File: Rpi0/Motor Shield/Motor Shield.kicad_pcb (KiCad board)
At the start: 2 copper layers, 29.8 x 64.8 mm, 37 parts, among them J1 Screw_Terminal_01x02, J3 Conn_02x01, J4 Screw_Terminal_01x02, J5 Screw_Terminal_01x02, J6 Conn_01x04_Female, J7 Conn_01x04_Female, Q1 Q_PMOS_GDSD, U1 IFX9201SG, U2 IFX9201SG, U3 PIC16F1509-ISS, U4 RPI0-Template, U6 ACT4060A

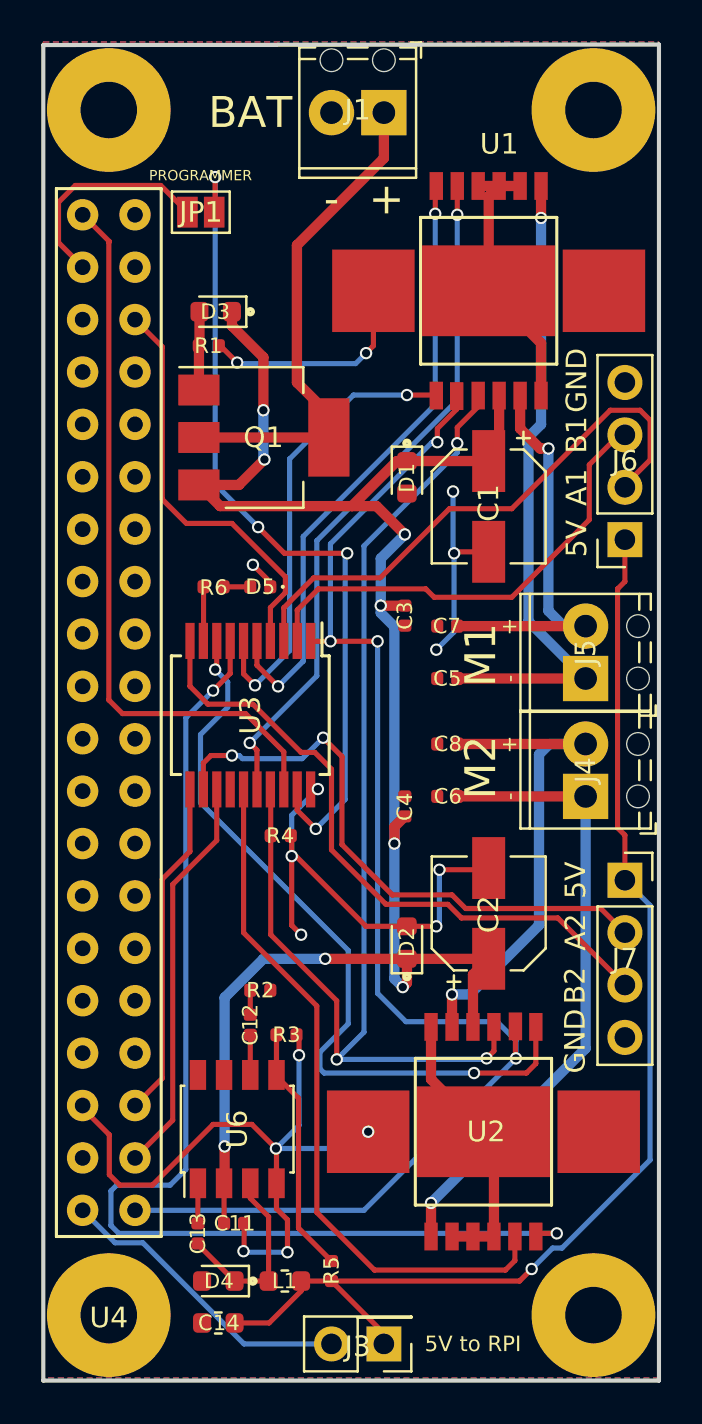
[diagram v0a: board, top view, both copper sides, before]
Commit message: Changed footprint
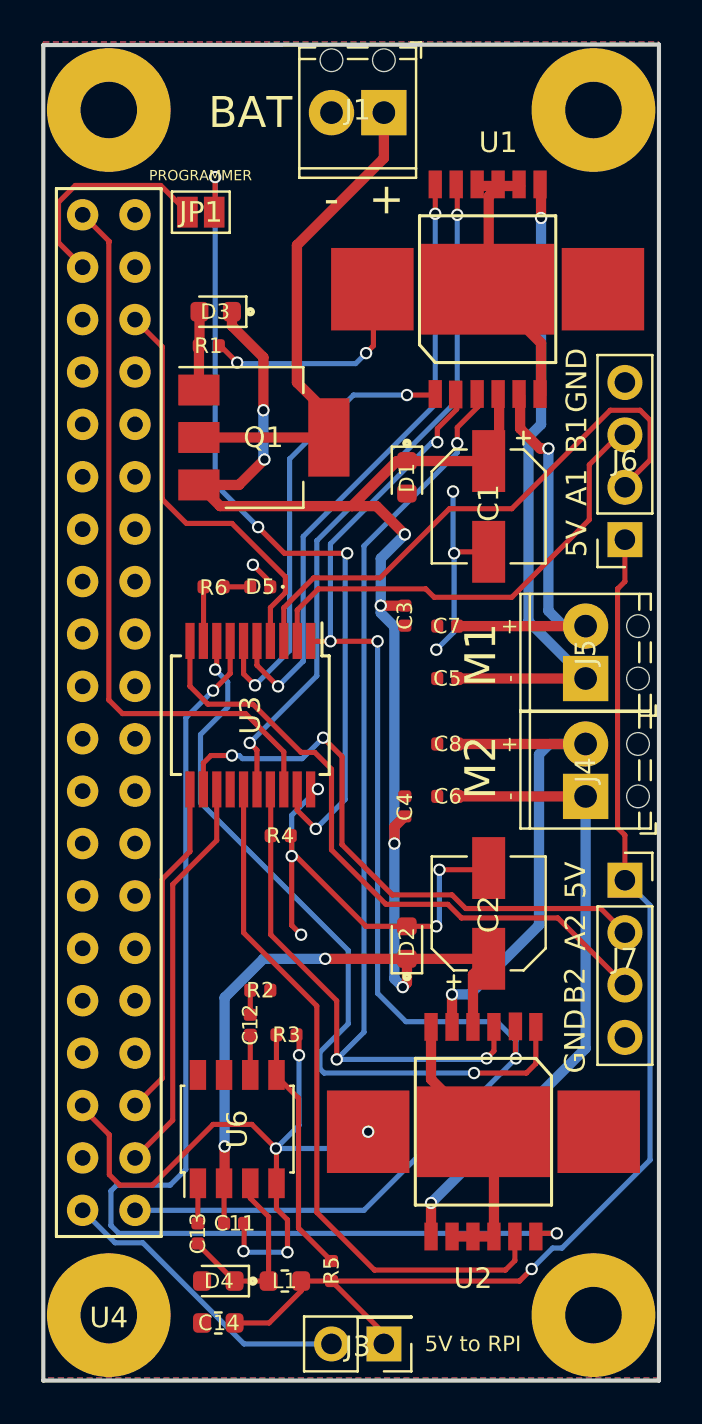
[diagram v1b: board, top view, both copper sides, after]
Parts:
- moved U1 0.09 mm to (163.8, 81.8)
